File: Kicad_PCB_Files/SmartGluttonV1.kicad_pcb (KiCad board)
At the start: 2 copper layers, 125.1 x 43.2 mm, 40 parts, among them J1 mDot breakout, J2 FLOW CONTROL, J3 mDot pin11-20 brkout, J4 mDot pin1-10 brkout, J5 USB_A, J6 USB_B, J7 GPS Connector, J8 Ultrasonic Conn, SW1 UART_PWR, SW2 Reset, U1 FT231XS, U2 MCP1700-3002E_TO92, U3 74LS04

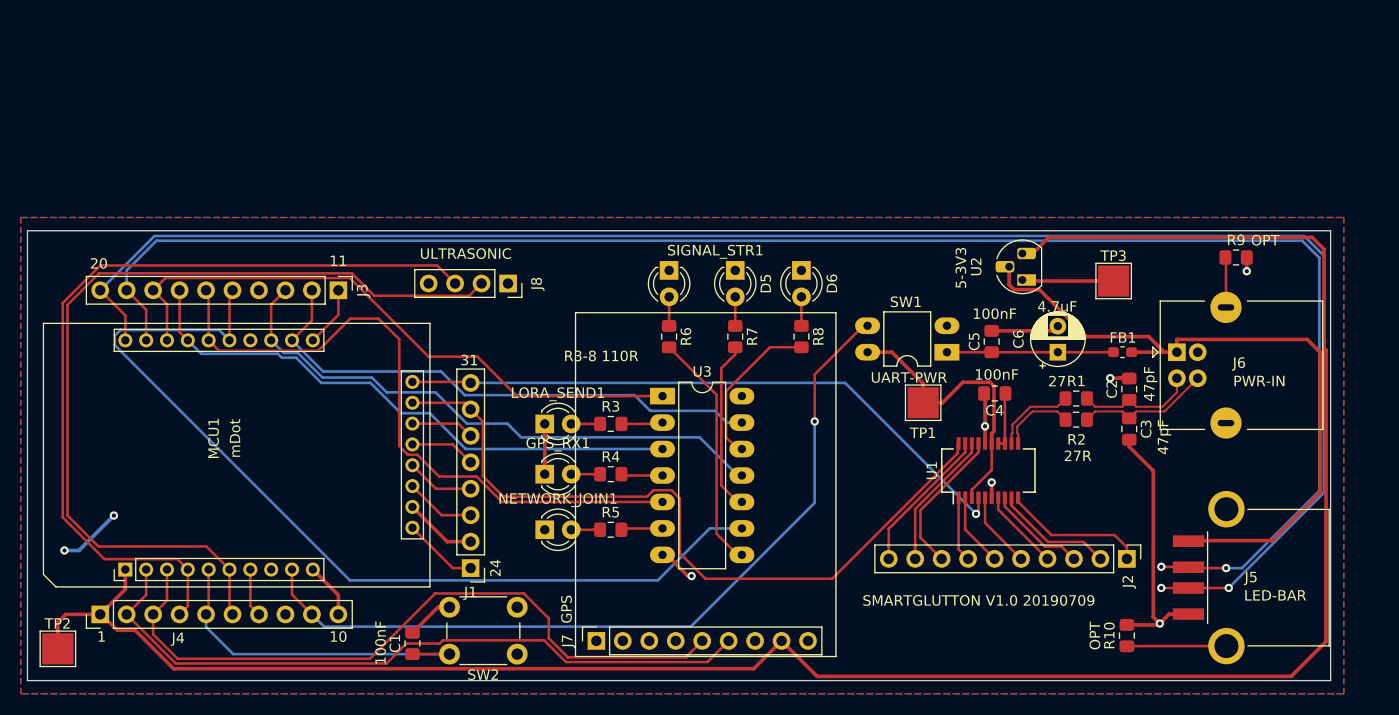
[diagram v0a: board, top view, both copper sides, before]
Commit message: Add files via upload
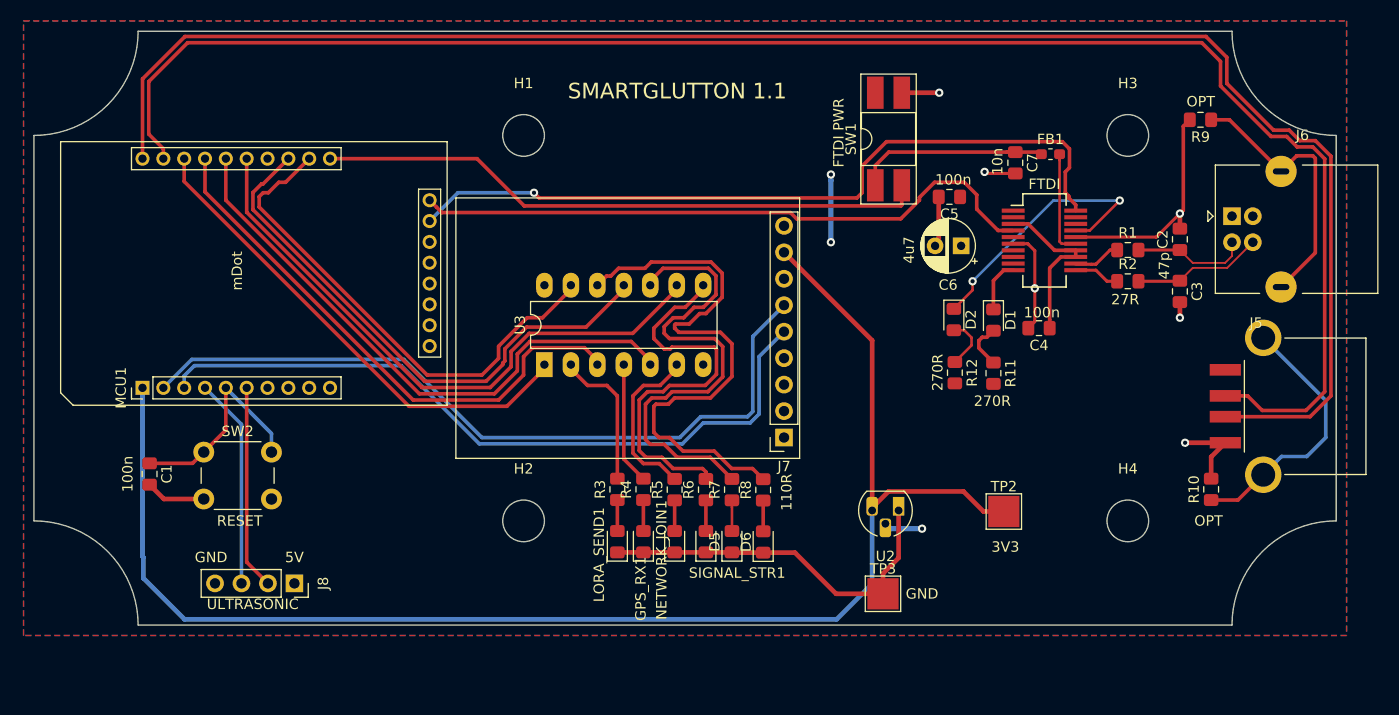
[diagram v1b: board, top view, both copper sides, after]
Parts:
- removed J1: mDot breakout, Connector_PinHeader_2.54mm:PinHeader_1x08_P2.54mm_Vertical
- removed J2: FLOW CONTROL, Connector_PinHeader_2.54mm:PinHeader_1x10_P2.54mm_Vertical
- removed J3: mDot pin11-20 brkout, Connector_PinHeader_2.54mm:PinHeader_1x10_P2.54mm_Vertical
- removed J4: mDot pin1-10 brkout, Connector_PinHeader_2.54mm:PinHeader_1x10_P2.54mm_Vertical
- removed TP1: TestPoint, TestPoint:TestPoint_Pad_3.0x3.0mm
- removed U1: FT231XS, Package_SO:SSOP-20_3.9x8.7mm_P0.635mm
- added C7: 10n, Capacitor_SMD:C_0805_2012Metric_Pad1.15x1.40mm_HandSolder, F.Cu at (174.2, 50.6)
- added D1: LED, LED_SMD:LED_0805_2012Metric_Pad1.15x1.40mm_HandSolder, F.Cu at (172.1, 65.7)
- added D2: LED, LED_SMD:LED_0805_2012Metric_Pad1.15x1.40mm_HandSolder, F.Cu at (168.3, 65.7)
- added FTDI: FT231XS, SmartGluttonV1:SSOP-20_3.9x8.7mm_P0.635mm_HandSolder, F.Cu at (177.0, 58.1)
- added H1: MountingHole, MountingHole:MountingHole_4mm, F.Cu at (127.0, 48.0)
- added H2: MountingHole, MountingHole:MountingHole_4mm, F.Cu at (127.0, 85.0)
- added H3: MountingHole, MountingHole:MountingHole_4mm, F.Cu at (185.0, 48.0)
- added H4: MountingHole, MountingHole:MountingHole_4mm, F.Cu at (185.0, 85.0)
- added R11: 270R, Resistor_SMD:R_0805_2012Metric_Pad1.15x1.40mm_HandSolder, F.Cu at (172.1, 70.8)
- added R12: 270R, Resistor_SMD:R_0805_2012Metric_Pad1.15x1.40mm_HandSolder, F.Cu at (168.4, 70.8)
- D5, D6, GPS_RX1, LORA_SEND1, NETWORK_JOIN1, SIGNAL_STR1: footprint LED_THT:LED_D3.0mm -> LED_SMD:LED_0805_2012Metric_Pad1.15x1.40mm_HandSolder
- SW1: value UART_PWR -> SW_DIP_x02; footprint Package_DIP:DIP-4_W7.62mm_LongPads -> Package_DIP:DIP-4_W8.89mm_SMDSocket_LongPads
- moved TP2 91.8 mm to (173.1, 84.1)
- moved TP3 37.3 mm to (161.5, 92.0)
- moved SW2 35.8 mm to (96.3, 78.4), turned to 0 degrees
- moved J8 35.3 mm to (105.0, 91.0)
- moved C1 30.0 mm to (91.1, 80.5), turned to 270 degrees
- moved J7 26.6 mm to (152.0, 77.0), turned to 180 degrees
- moved D6 26.3 mm to (150.0, 87.0), turned to 90 degrees
- moved SIGNAL_STR1 26.3 mm to (144.5, 87.0), turned to 90 degrees
- moved D5 26.0 mm to (147.0, 87.0), turned to 90 degrees
- moved U2 25.1 mm to (163.0, 84.0), turned to 180 degrees
- moved SW1 21.2 mm to (162.0, 48.3), turned to 90 degrees
- moved FB1 20.2 mm to (177.6, 49.8), turned to 0 degrees
- moved MCU1 17.5 mm to (119.8, 74.0)
- moved J5 16.8 mm to (195.9, 74.0)
- moved R10 16.2 mm to (193.0, 82.0)
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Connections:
- C5 pad 1: Net-(C5-Pad1) -> +5V
- C6 pad 1: Net-(C5-Pad1) -> +5V
- FB1 pad 1: +5V -> Net-(C7-Pad1)
- FB1 pad 2: Net-(C5-Pad1) -> Net-(FB1-Pad2)
- MCU1 pad 11: Net-(J3-Pad1) -> PA_7
- MCU1 pad 9: Net-(J4-Pad9) -> Net-(MCU1-Pad9)
- SW1 pad 1: Net-(C5-Pad1) -> Net-(C7-Pad1)
- SW1 pad 2: GND -> PA_7
- SW1 pad 3: Net-(J4-Pad9) -> GND
- SW1 pad 4: Net-(SW1-Pad4) -> +5V
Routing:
- net Net-(J4-Pad9): track 78.1 -> 0.00 mm, vias 1 -> 0
- net Net-(J8-Pad2): track 84.7 -> 19.6 mm
- net +5V: track 73.1 -> 10.2 mm, vias 2 -> 3
- net +3V3: track 203.8 -> 141.0 mm
- net Net-(J8-Pad3): track 79.2 -> 20.2 mm
- net PA_7: track 0.00 -> 58.7 mm
- net Net-(R8-Pad2): track 15.4 -> 54.4 mm
- net Net-(R7-Pad2): track 16.5 -> 47.0 mm
- net LED4: track 89.1 -> 58.6 mm
- net Net-(SW1-Pad4): track 27.8 -> 0.00 mm
- net Net-(D2-Pad1): track 0.00 -> 26.6 mm, vias 0 -> 2
- net Net-(J6-Pad5): track 4.82 -> 26.5 mm
- net GND: track 75.3 -> 94.2 mm
- net Net-(C7-Pad1): track 0.00 -> 18.5 mm
- net Net-(C5-Pad1): track 16.0 -> 0.00 mm
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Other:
- board size 125.1 x 43.2 mm -> 125 x 57 mm
- net class Default: trace_width 0.25 -> 0.35
- net class SSOP added: clearance 0.2, trace_width 0.25, via_dia 0.8, via_drill 0.4
- net class USB: clearance 0.2 -> 0.18; trace_width 0.25 -> 0.3
- board text added: "100n"
- board text added: "10n"
- board text added: "110R"
- board text added: "270R"
- board text added: "3V3"
- board text added: "47p"
- board text added: "4u7"
- board text added: "5V"
- board text added: "FTDI PWR"
- board text added: "GND"
- board text added: "RESET"
- board text added: "SMARTGLUTTON 1.1"
- board text removed: "1"
- board text removed: "10"
- board text removed: "100nF"
- board text removed: "11"
- board text removed: "20"
- board text removed: "24"
- board text removed: "27"
- board text removed: "31"
- board text removed: "4.7uF"
- board text removed: "47pF"
- board text removed: "5-3V3"
- board text removed: "GPS"
- board text removed: "LED-BAR"
- board text removed: "PWR-IN"
- board text removed: "R3-8 110R"
- board text removed: "SMARTGLUTTON V1.0 20190709"
- board text removed: "UART-PWR"

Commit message: Add files via upload
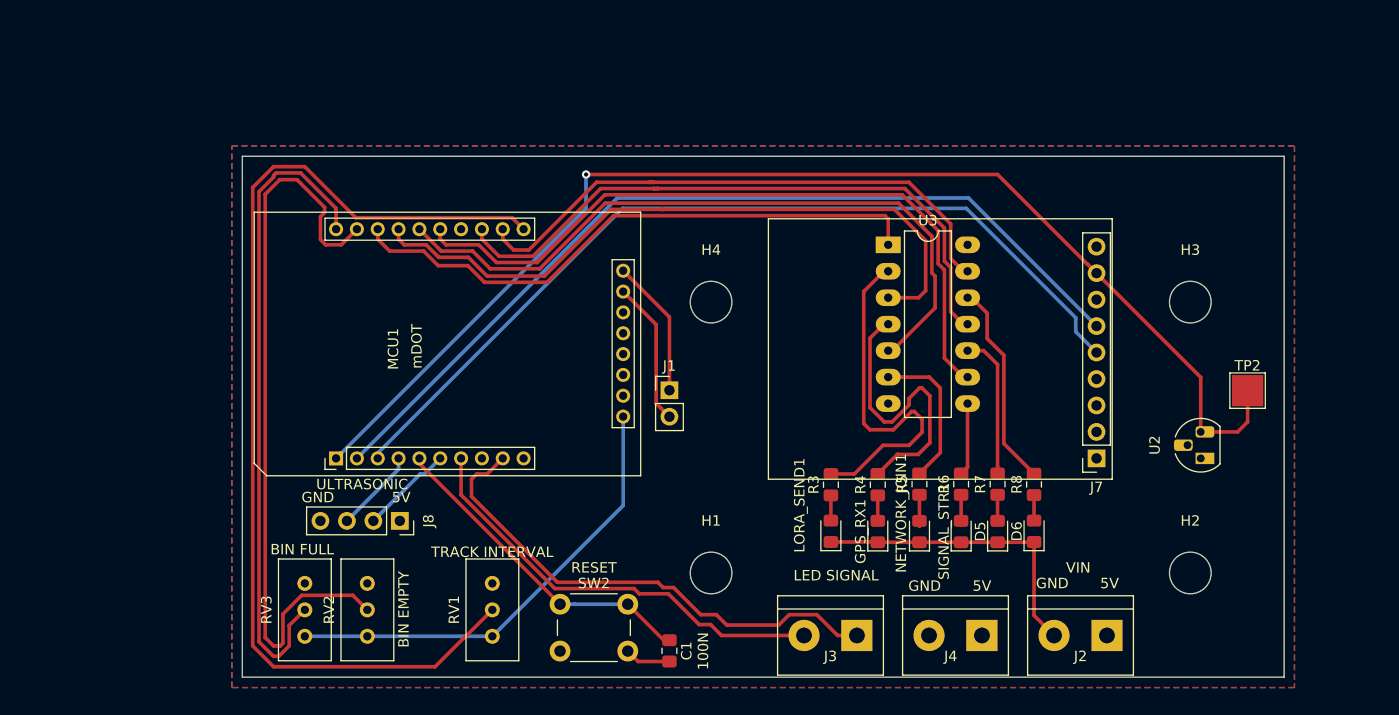
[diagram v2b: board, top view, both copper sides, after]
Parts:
- removed C2, C3: 47pF, Capacitor_SMD:C_0805_2012Metric_Pad1.15x1.40mm_HandSolder
- removed C4, C5: 100nF, Capacitor_SMD:C_0805_2012Metric_Pad1.15x1.40mm_HandSolder
- removed C6: 4.7uF, Capacitor_THT:CP_Radial_D5.0mm_P2.50mm
- removed C7: 10n, Capacitor_SMD:C_0805_2012Metric_Pad1.15x1.40mm_HandSolder
- removed D1, D2: LED, LED_SMD:LED_0805_2012Metric_Pad1.15x1.40mm_HandSolder
- removed FB1: 47@100MHz, Inductor_SMD:L_0603_1608Metric_Pad1.05x0.95mm_HandSolder
- removed FTDI: FT231XS, SmartGluttonV1:SSOP-20_3.9x8.7mm_P0.635mm_HandSolder
- removed J5: USB_A, SmartGluttonV1:USB_A_FCI_87583_Horizontal
- removed J6: USB_B, SmartGluttonV1:USB_B_Molex_USB-67068-xx1x_StraightTab_Horizontal
- removed R1, R2: 27, Resistor_SMD:R_0805_2012Metric_Pad1.15x1.40mm_HandSolder
- removed R10, R9: 0R OPT, Resistor_SMD:R_0805_2012Metric_Pad1.15x1.40mm_HandSolder
- removed R11, R12: 270R, Resistor_SMD:R_0805_2012Metric_Pad1.15x1.40mm_HandSolder
- removed SW1: SW_DIP_x02, Package_DIP:DIP-4_W8.89mm_SMDSocket_LongPads
- removed TP3: TestPoint, TestPoint:TestPoint_Pad_3.0x3.0mm
- added J1: Conn_01x02_Female, Connector_PinHeader_2.54mm:PinHeader_1x02_P2.54mm_Vertical, F.Cu at (141.0, 72.5)
- added J2: Screw_Terminal_01x02, TerminalBlock:TerminalBlock_bornier-2_P5.08mm, F.Cu at (183.0, 96.0)
- added J3: Screw_Terminal_01x02, TerminalBlock:TerminalBlock_bornier-2_P5.08mm, F.Cu at (159.0, 96.0)
- added J4: Screw_Terminal_01x02, TerminalBlock:TerminalBlock_bornier-2_P5.08mm, F.Cu at (171.0, 96.0)
- added RV1: R_POT, Potentiometer_THT:Potentiometer_Bourns_3296W_Vertical, F.Cu at (124.0, 91.0)
- added RV2: R_POT, Potentiometer_THT:Potentiometer_Bourns_3296W_Vertical, F.Cu at (112.0, 91.0)
- added RV3: R_POT, Potentiometer_THT:Potentiometer_Bourns_3296W_Vertical, F.Cu at (106.0, 91.0)
- moved H2 64.2 mm to (191.0, 90.0)
- moved C1 52.7 mm to (141.0, 97.5)
- moved H1 45.7 mm to (145.0, 90.0)
- moved H4 45.2 mm to (145.0, 64.0)
- moved SW2 37.2 mm to (130.5, 93.0)
- moved U3 34.9 mm to (162.0, 58.5), turned to 0 degrees
- moved J7 30.1 mm to (182.0, 79.0)
- moved U2 29.4 mm to (192.0, 79.0), turned to 90 degrees
- moved TP2 26.1 mm to (196.5, 72.5)
- moved D6 26.0 mm to (176.0, 86.0)
- moved R8 26.0 mm to (176.0, 81.5)
- moved D5 25.5 mm to (172.5, 86.0)
- moved R7 25.5 mm to (172.5, 81.5)
- moved SIGNAL_STR1 24.5 mm to (169.0, 86.0)
- moved R6 24.5 mm to (169.0, 81.5)
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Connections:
- MCU1 pad 11: PA_7 -> Net-(MCU1-Pad11)
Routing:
- net Net-(MCU1-Pad20): track 163.6 -> 62.8 mm
- net Net-(MCU1-Pad11): track 0.00 -> 99.4 mm
- net Net-(MCU1-Pad19): track 161.6 -> 71.9 mm
- net GND: track 94.2 -> 33.7 mm, vias 6 -> 0
- net Net-(J1-Pad2): track 73.3 -> 13.8 mm, vias 1 -> 0
- net PA_7: track 58.7 -> 0.00 mm
- net Net-(J3-Pad1): track 0.00 -> 48.8 mm
- net Net-(J1-Pad1): track 61.1 -> 13.3 mm
- net Net-(MCU1-Pad24): track 0.00 -> 44.3 mm
- net Net-(J3-Pad2): track 0.00 -> 42.0 mm
- net Net-(R8-Pad2): track 54.4 -> 19.8 mm
- net Net-(R7-Pad2): track 47.0 -> 13.9 mm
- net Net-(R6-Pad2): track 37.9 -> 6.97 mm
- net Net-(D2-Pad1): track 26.6 -> 0.00 mm, vias 2 -> 0
- net Net-(J6-Pad5): track 26.5 -> 0.00 mm
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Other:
- board size 125 x 57 mm -> 100 x 50 mm
- net class Default: clearance 0.2 -> 0.25
- net class PWR: clearance 0.2 -> 0.25
- net class SSOP removed
- net class USB removed
- rule trace_clearance: 0.2 -> 0.25
- board text added: "100N"
- board text added: "BIN EMPTY"
- board text added: "BIN FULL"
- board text added: "LED SIGNAL"
- board text added: "TRACK INTERVAL"
- board text added: "VIN"
- board text added: "mDOT"
- board text removed: "100n"
- board text removed: "10n"
- board text removed: "110R"
- board text removed: "270R"
- board text removed: "27R"
- board text removed: "3V3"
- board text removed: "47p"
- board text removed: "4u7"
- board text removed: "FTDI PWR"
- board text removed: "OPT"
- board text removed: "SMARTGLUTTON 1.1"
- board text removed: "mDot"
